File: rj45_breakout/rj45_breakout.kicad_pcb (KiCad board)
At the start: 2 copper layers, 48.8 x 19.8 mm, 3 parts, among them J1 RJ45_LED, J2 CONN_01X04, J3 CONN_01X05

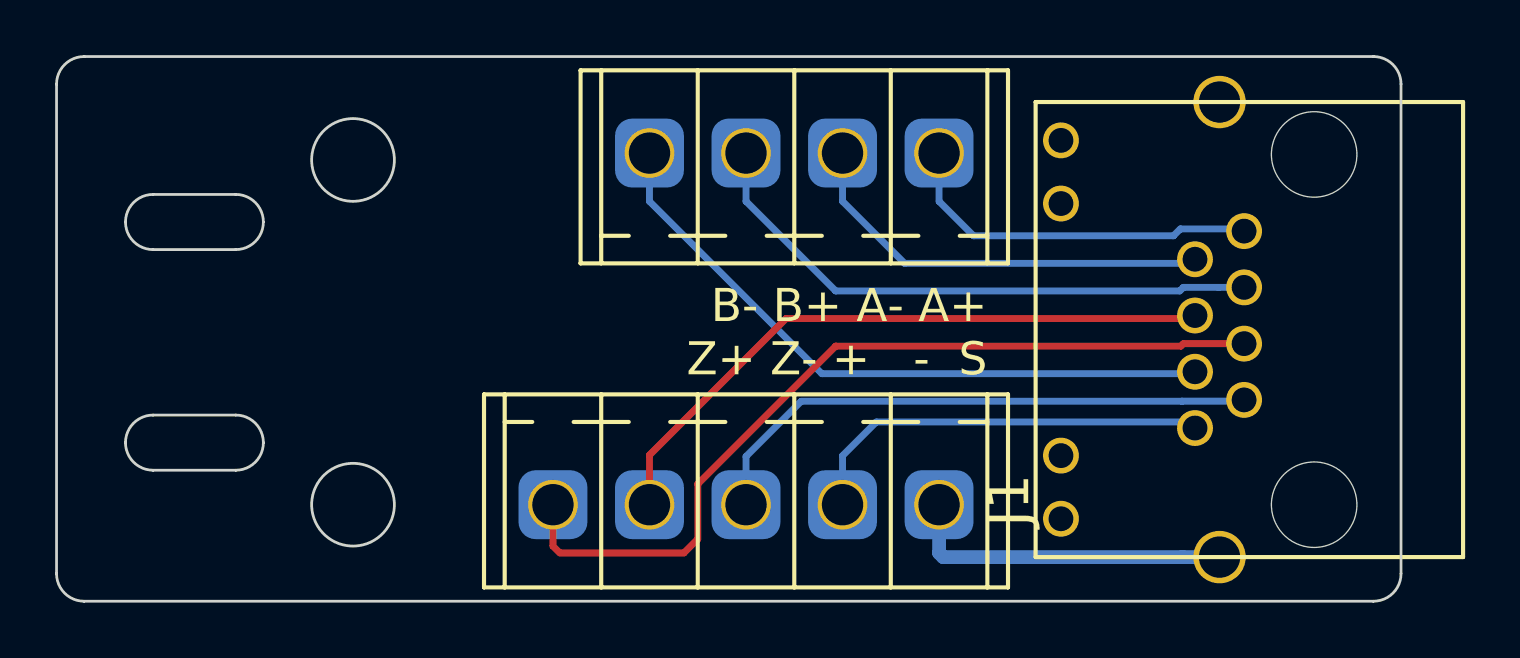
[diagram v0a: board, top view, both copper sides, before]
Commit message: hw
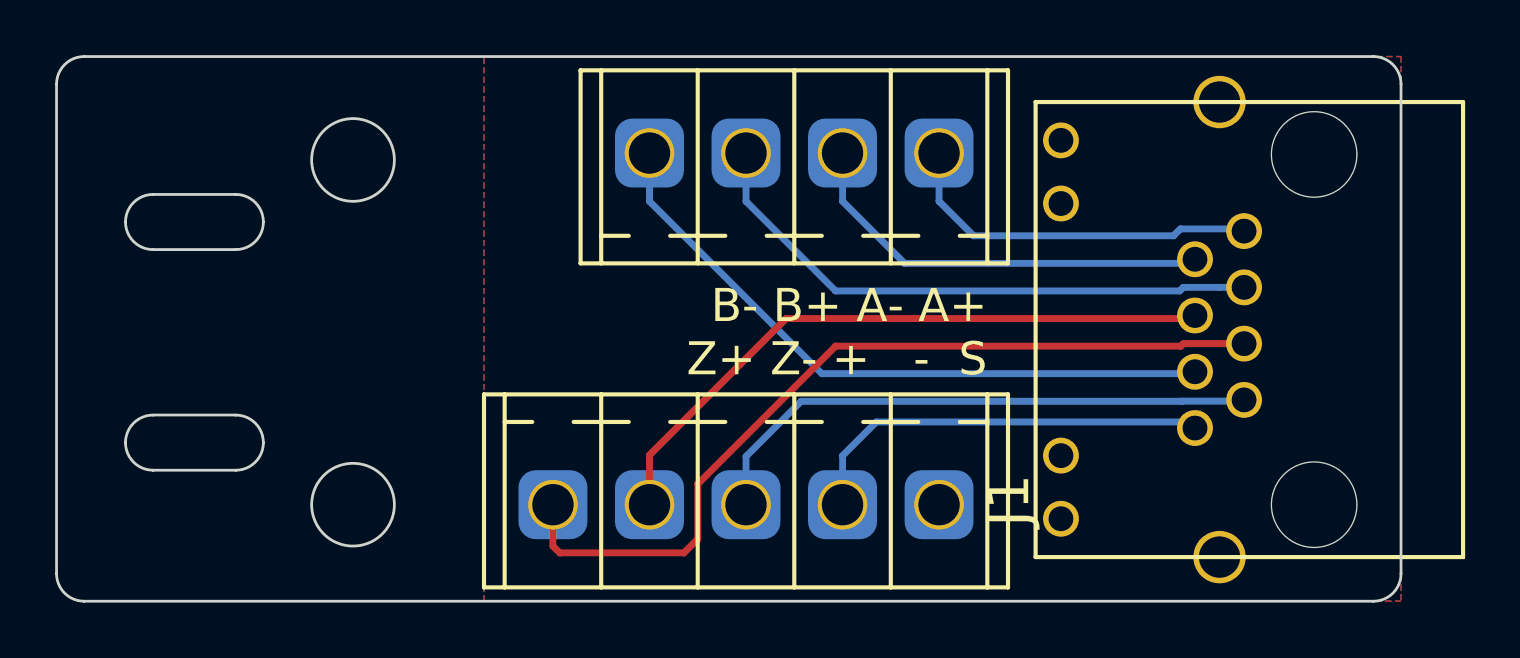
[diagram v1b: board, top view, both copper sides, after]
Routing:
- net Net-(J1-Pad13): track 12.0 -> 0.00 mm
- added copper zone on B.Cu, net Net-(J1-Pad13)
- added copper zone on F.Cu, net Net-(J1-Pad13)
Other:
- net class Default: clearance 0.2 -> 0.15; via_dia 0.8 -> 0.6; via_drill 0.4 -> 0.3
- rule trace_clearance: 0.2 -> 0.15
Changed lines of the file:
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@@
     (thickness 1.6)
     (drawings 24)
-    (tracks 47)
+    (tracks 43)
     (zones 0)
     (modules 3)
@@
   (setup
     (last_trace_width 0.25)
-    (trace_clearance 0.2)
-    (zone_clearance 0.508)
+    (trace_clearance 0.15)
+    (zone_clearance 0.2)
     (zone_45_only no)
     (trace_min 0.2)
-    (via_size 0.8)
-    (via_drill 0.4)
+    (via_size 0.6)
+    (via_drill 0.3)
     (via_min_size 0.4)
     (via_min_drill 0.3)
@@
   (net 9 "Net-(J1-Pad8)")
   (net_class Default "This is the default net class."
-    (clearance 0.2)
+    (clearance 0.15)
     (trace_width 0.25)
-    (via_dia 0.8)
-    (via_drill 0.4)
+    (via_dia 0.6)
+    (via_drill 0.3)
     (uvia_dia 0.3)
     (uvia_drill 0.1)
     (add_net "Net-(J1-Pad1)")
-    (add_net "Net-(J1-Pad10)")
-    (add_net "Net-(J1-Pad11)")
-    (add_net "Net-(J1-Pad12)")
     (add_net "Net-(J1-Pad13)")
     (add_net "Net-(J1-Pad2)")
@@
     (add_net "Net-(J1-Pad7)")
     (add_net "Net-(J1-Pad8)")
-    (add_net "Net-(J1-Pad9)")
   )
   (module stmbl:RM3.5_1x5_UP (layer F.Cu)
@@
     (effects (font (size 1.2 1.2) (thickness 0.25)) (justify right))
   )
-  (segment (start 125.076498 71.9) (end 126.42 71.9) (width 0.5) (layer B.Cu) (net 1))
-  (segment (start 116.25 70) (end 116.25 71.75) (width 0.5) (layer B.Cu) (net 1))
-  (segment (start 116.25 71.75) (end 116.4 71.9) (width 0.5) (layer B.Cu) (net 1))
-  (segment (start 116.4 71.9) (end 125.076498 71.9) (width 0.5) (layer B.Cu) (net 1))
   (segment (start 127.23 60) (end 127.31 60.08) (width 0.25) (layer B.Cu) (net 2))
   (segment (start 124.75 60.25) (end 125 60) (width 0.25) (layer B.Cu) (net 2))
@@
   (segment (start 112.75 68.225) (end 113.975 67) (width 0.25) (layer B.Cu) (net 9))
   (segment (start 112.75 70) (end 112.75 68.225) (width 0.25) (layer B.Cu) (net 9))
+  (zone (net 1) (net_name "Net-(J1-Pad13)") (layer F.Cu) (hatch edge 0.508)
+    (connect_pads (clearance 0.2))
+    (min_thickness 0.2)
+    (fill yes (arc_segments 32) (thermal_gap 0.2) (thermal_bridge_width 0.25))
+    (polygon
+      (pts
+        (xy 133 53.75) (xy 133 73.5) (xy 99.75 73.5) (xy 99.75 53.75)
+      )
+    )
+  )
+  (zone (net 1) (net_name "Net-(J1-Pad13)") (layer B.Cu) (hatch edge 0.508)
+    (connect_pads (clearance 0.2))
+    (min_thickness 0.2)
+    (fill yes (arc_segments 32) (thermal_gap 0.2) (thermal_bridge_width 0.25))
+    (polygon
+      (pts
+        (xy 133 53.75) (xy 133 73.5) (xy 99.75 73.5) (xy 99.75 53.75)
+      )
+    )
+  )
 )
